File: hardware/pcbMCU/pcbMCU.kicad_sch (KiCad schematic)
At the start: 20 parts

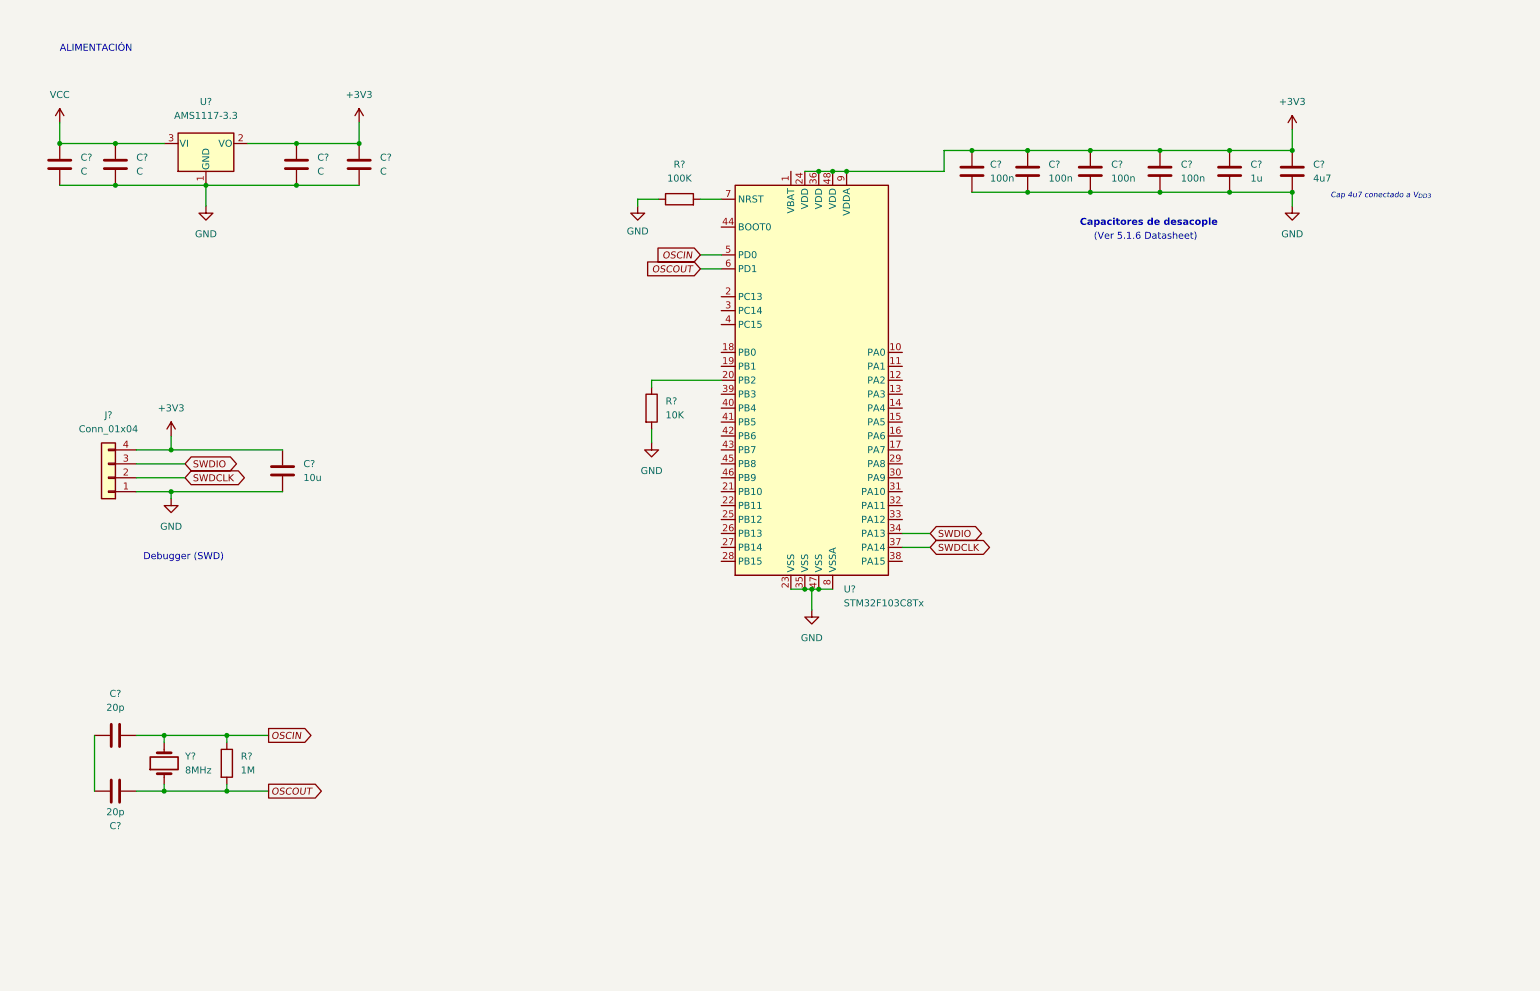
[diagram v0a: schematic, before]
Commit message: Regulación de alimentación de entrada
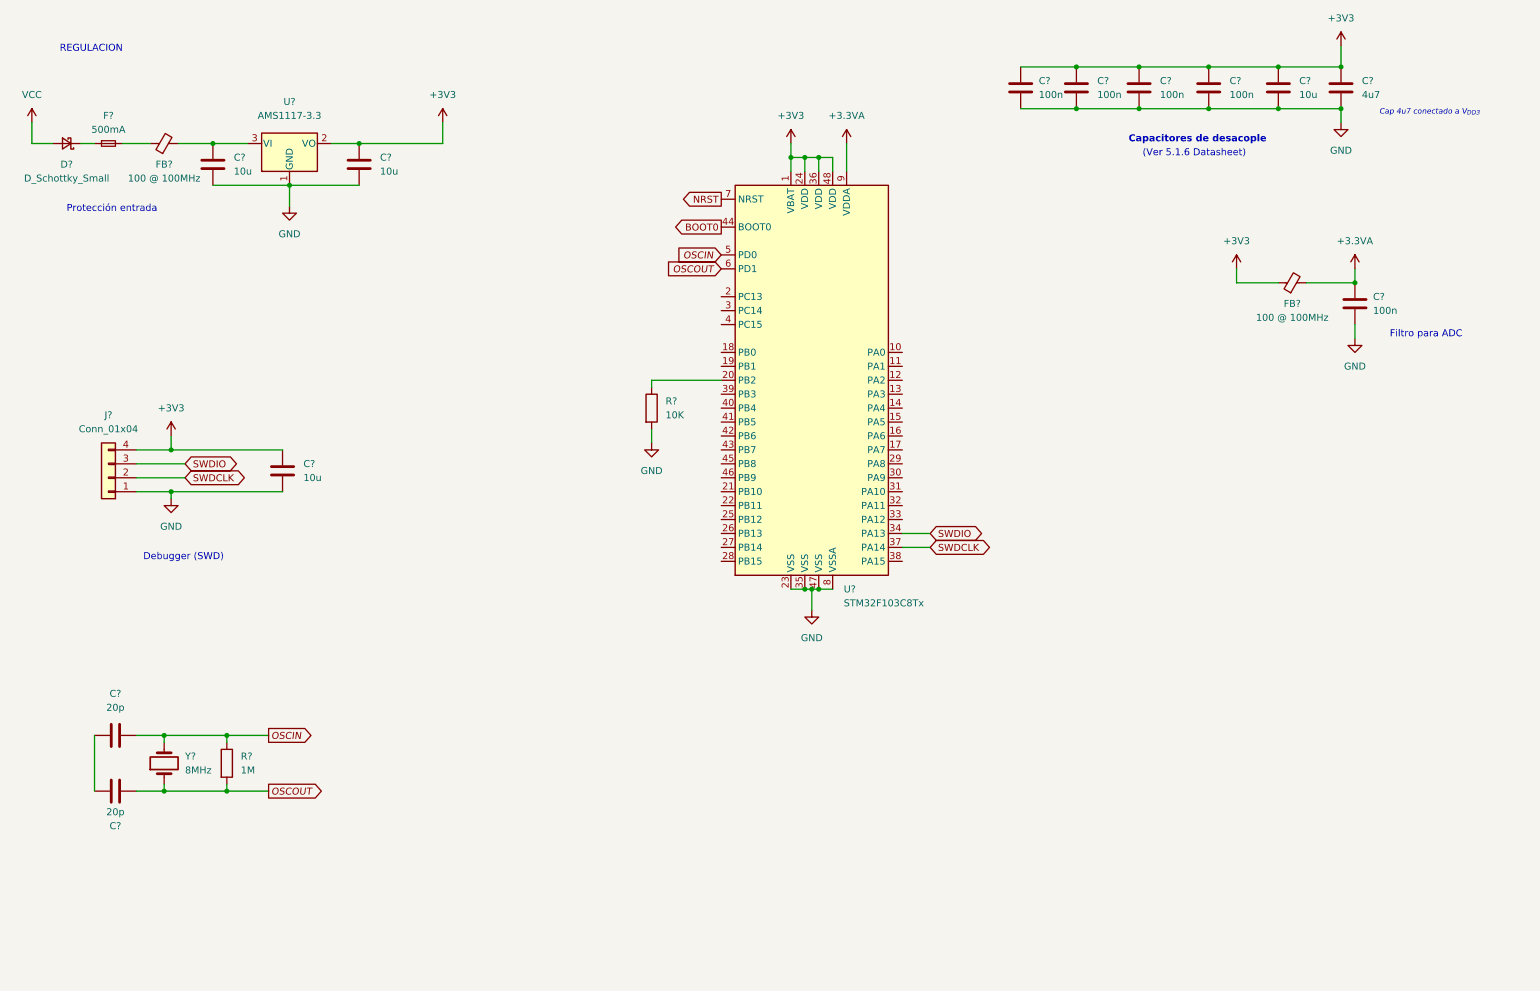
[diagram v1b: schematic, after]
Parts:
- removed C? (x2): C, symbol Device:C
- removed R?: 100K, symbol Device:R
- added C?: 100n, symbol Device:C
- added D?: D_Schottky_Small, symbol Device:D_Schottky_Small
- added F?: 500mA, symbol Device:Fuse_Small
- added FB? (x2): 100 @ 100MHz, symbol Device:FerriteBead_Small
- C? (x2): value C -> 10u
- C?: value 1u -> 10u
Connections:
- net +3V3: now also U?.1 (VBAT), FB?.1; no longer U?.9 (VDDA)
- net GND: now also C?.2
- net VCC: now also D?.2 (A); no longer C?.1, U?.3 (VI)
- net NRST: now reaches U?.7 (NRST)
- net BOOT0: now reaches U?.44 (BOOT0)
- new net: D?.1 (K), F?.1
- new net: C?.1, FB?.2, U?.3 (VI)
- new net: F?.2, FB?.1
- new net +3.3VA: C?.1, FB?.2, U?.9 (VDDA)
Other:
- note added: "Filtro para ADC"
- note added: "Protección entrada"
- note added: "REGULACION"
- note removed: "ALIMENTACIÓN"
- moved on the sheet: C?, U?

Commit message: Rev1 terminada
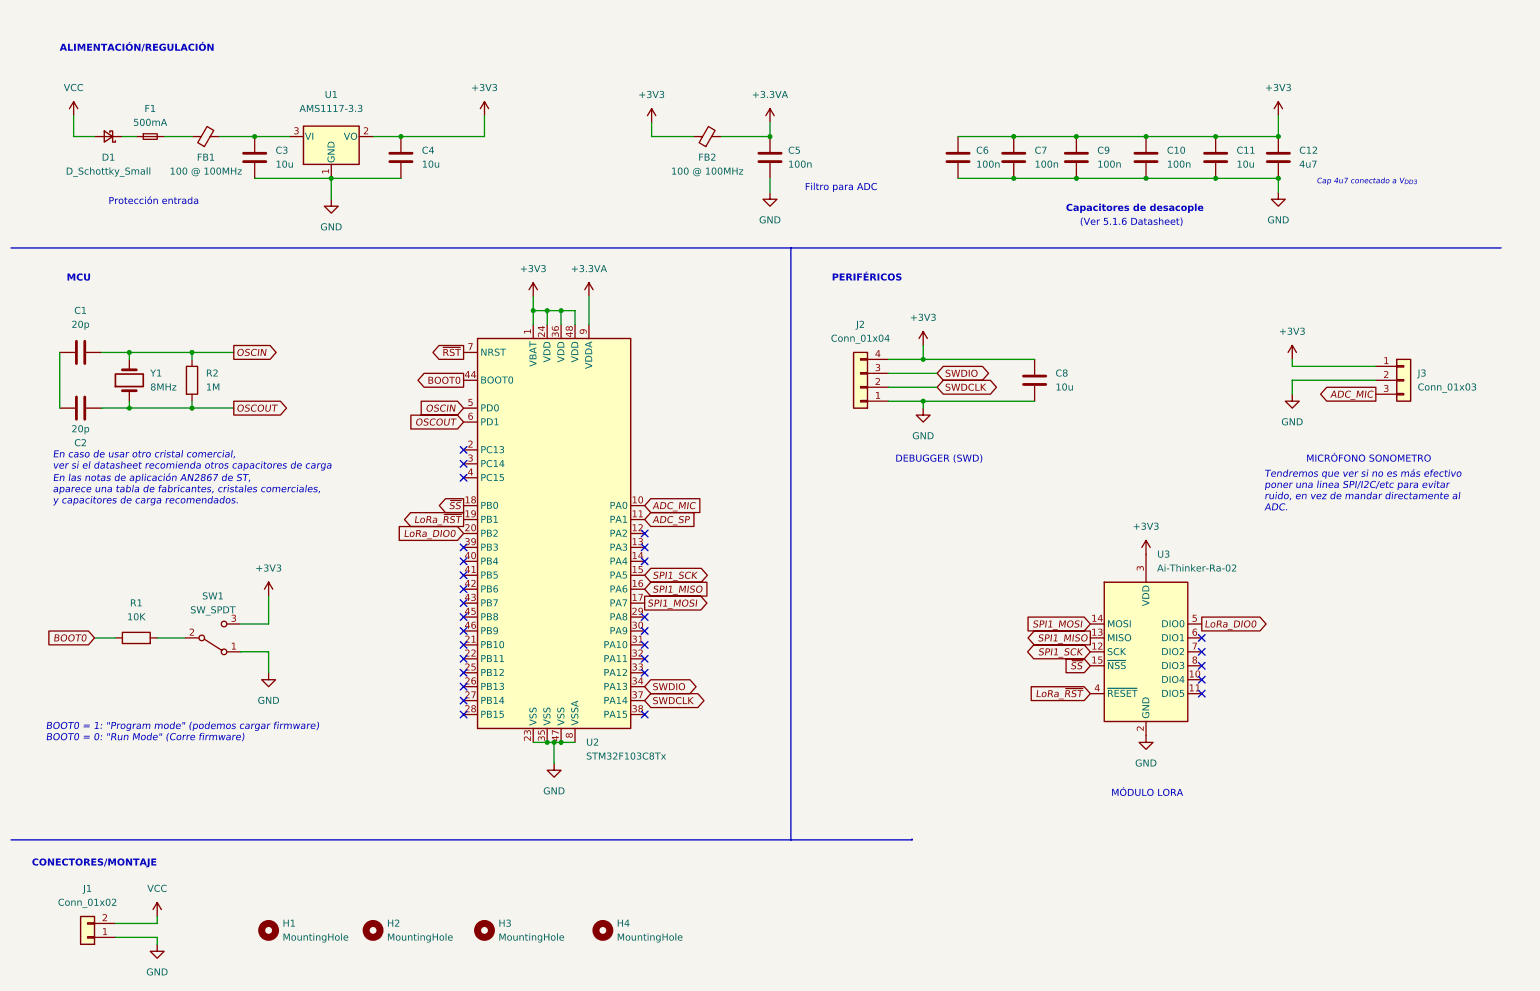
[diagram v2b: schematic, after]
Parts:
- removed R?: 10K, symbol Device:R
- added H1, H2, H3, H4: MountingHole, symbol Mechanical:MountingHole
- added J1: Conn_01x02, symbol Connector_Generic:Conn_01x02
- added J3: Conn_01x03, symbol Connector_Generic:Conn_01x03
- added R1: 10K, symbol Device:R
- added SW1: SW_SPDT, symbol Switch:SW_SPDT
- added U3: Ai-Thinker-Ra-02, RF_Module:Ai-Thinker-Ra-01-LoRa, symbol RF_Module:Ai-Thinker-Ra-02
- gave numbers to parts that had none: 21
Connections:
- net +3V3: now also J3.1 (Pin_1), SW1.3 (C), U3.3 (VDD)
- net BOOT0: now also R1.1
- net GND: now also J1.1 (Pin_1), J3.2 (Pin_2), SW1.1 (A), U3.1 (GND), U3.16 (GND), U3.2 (GND), U3.9 (GND)
- net VCC: now also J1.2 (Pin_2)
- net LoRa_DIO0: now reaches U2.20 (PB2)
- net LoRa_DIO0: now also U3.5 (DIO0)
- net ADC_MIC: now reaches U2.10 (PA0)
- net ADC_MIC: now also J3.3 (Pin_3)
- net ADC_SP: now reaches U2.11 (PA1)
- net SPI1_SCK: now reaches U2.15 (PA5)
- net SPI1_SCK: now also U3.12 (SCK)
- net SPI1_MISO: now reaches U2.16 (PA6)
- net SPI1_MISO: now also U3.13 (MISO)
- net SPI1_MOSI: now reaches U2.17 (PA7)
- net SPI1_MOSI: now also U3.14 (MOSI)
- net ~{SS}: now reaches U2.18 (PB0)
- net ~{SS}: now also U3.15 (~{NSS})
- net LoRa_~{RST}: now reaches U2.19 (PB1)
- net LoRa_~{RST}: now also U3.4 (~{RESET})
- net NRST renamed ~{RST}
- new net: R1.2, SW1.2 (B)
- no-connect marks 0 -> 30
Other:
- note added: "ALIMENTACIÓN/REGULACIÓN"
- note added: "BOOT0 = 1: "Program mode" (podemos cargar firmware) BOOT0 = 0: "Run Mode" (Corre firmware)"
- note added: "CONECTORES/MONTAJE"
- note added: "DEBUGGER (SWD)"
- note added: "En caso de usar otro cristal comercial, ver si el datasheet recomienda otros capacitores de carga"
- note added: "En las notas de aplicación AN2867 de ST, aparece una tabla de fabricantes, cristales comerciales, y capacitores de carga recomendados."
- note added: "MCU"
- note added: "MICRÓFONO SONOMETRO"
- note added: "MÓDULO LORA"
- note added: "PERIFÉRICOS"
- note added: "Tendremos que ver si no es más efectivo poner una linea SPI/I2C/etc para evitar ruido, en vez de mandar directamente al ADC."
- note removed: "Debugger (SWD)"
- note removed: "REGULACION"
- company: (none) -> Franco Montanari, Dante Conti, Maximiliano Gonzales
- title: (none) -> Sensor partículas IoT
- moved on the sheet: C1, C10, C11, C12, C2, C3, C4, C5, C6, C7, C8, C9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
